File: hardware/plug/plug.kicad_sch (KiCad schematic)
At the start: 33 parts, among them J101 Cortex, J102 DX07S016JA3, SW101 SKSG, U101 ATSAMD51J, U102 TPS78433QWDRBRQ1, Y101 32k768

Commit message: Good Bye Imperial
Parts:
- C101, C102: footprint V2_Capacitor_SMD:C_0603 -> V2_Capacitor_SMD:C_1608; symbol V2_Capacitor:0603_18p -> V2_Capacitor:1608_18p
- C103, C105, C106, C107, C108, C109: footprint V2_Capacitor_SMD:C_0603 -> V2_Capacitor_SMD:C_1608; symbol V2_Capacitor:0603_0u1 -> V2_Capacitor:1608_0u1
- C104: footprint V2_Capacitor_SMD:C_0603 -> V2_Capacitor_SMD:C_1608; symbol V2_Capacitor:0603_10u -> V2_Capacitor:1608_10u
- C110, C111: footprint V2_Capacitor_SMD:C_0805 -> V2_Capacitor_SMD:C_2012; symbol V2_Capacitor:0805_10u -> V2_Capacitor:2012_10u
- D103: footprint V2_LED:LED_0603 -> V2_LED:LED_1608; symbol V2_LED:0603_Orange -> V2_LED:1608_Orange
- R101: footprint V2_Resistor_SMD:R_0603 -> V2_Resistor_SMD:R_1608; symbol V2_Resistor:0603_100k -> V2_Resistor:1608_100k
- R102: footprint V2_Resistor_SMD:R_0603 -> V2_Resistor_SMD:R_1608; symbol V2_Resistor:0603_330R -> V2_Resistor:1608_330R
- R103, R104: footprint V2_Resistor_SMD:R_0603 -> V2_Resistor_SMD:R_1608; symbol V2_Resistor:0603_5k1 -> V2_Resistor:1608_5k1

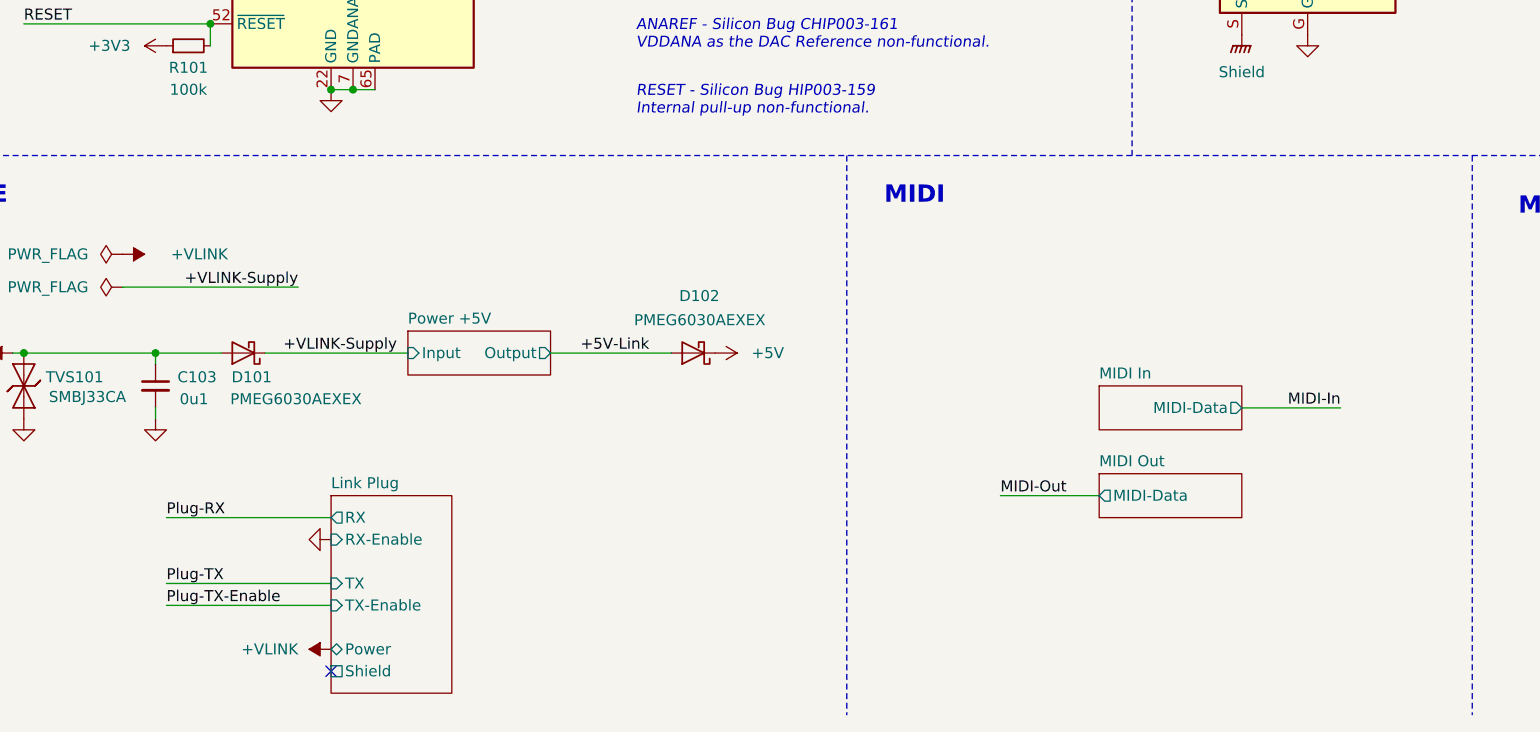
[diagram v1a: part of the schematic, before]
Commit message: Refresh
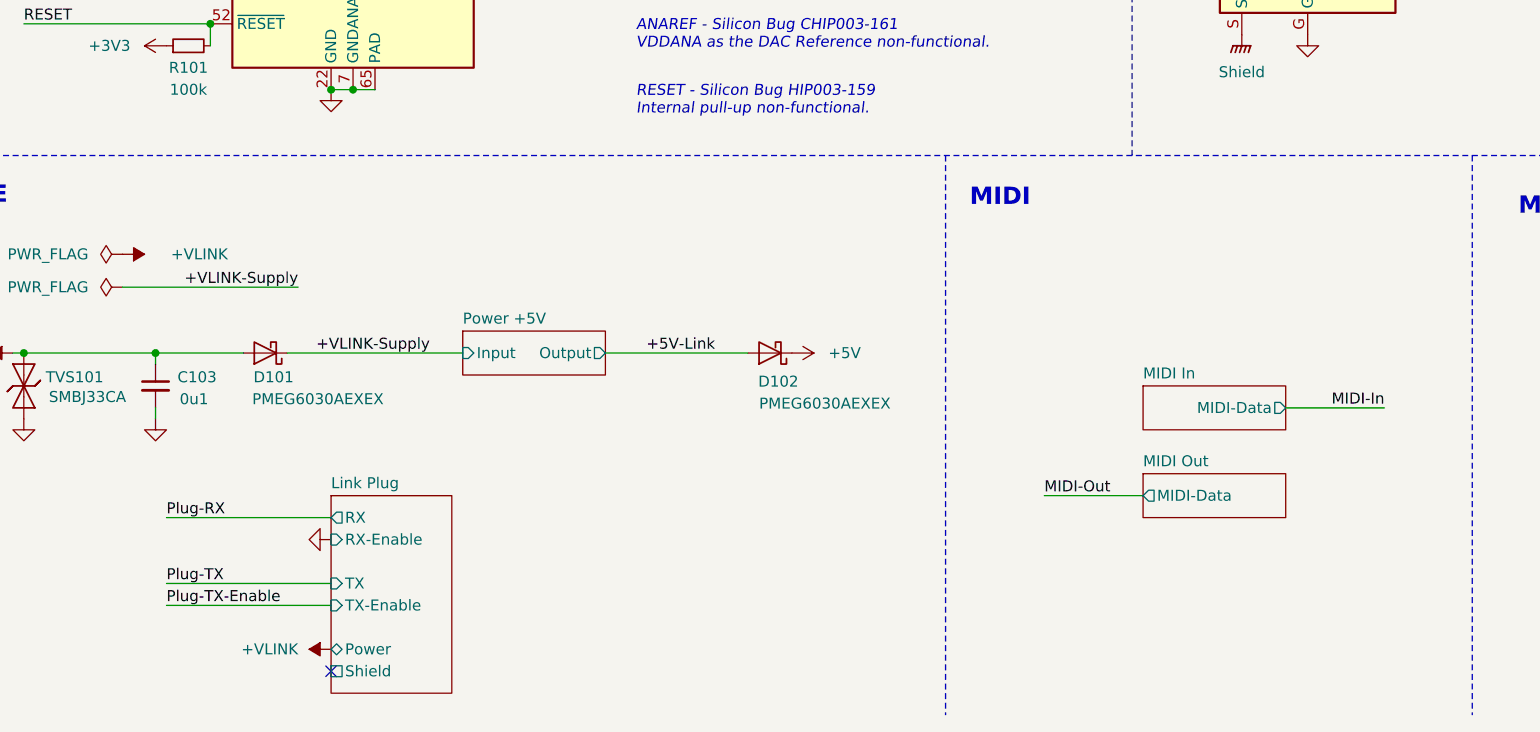
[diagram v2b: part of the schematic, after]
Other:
- moved on the sheet: D101, D102
